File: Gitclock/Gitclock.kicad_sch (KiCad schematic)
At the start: 6 parts

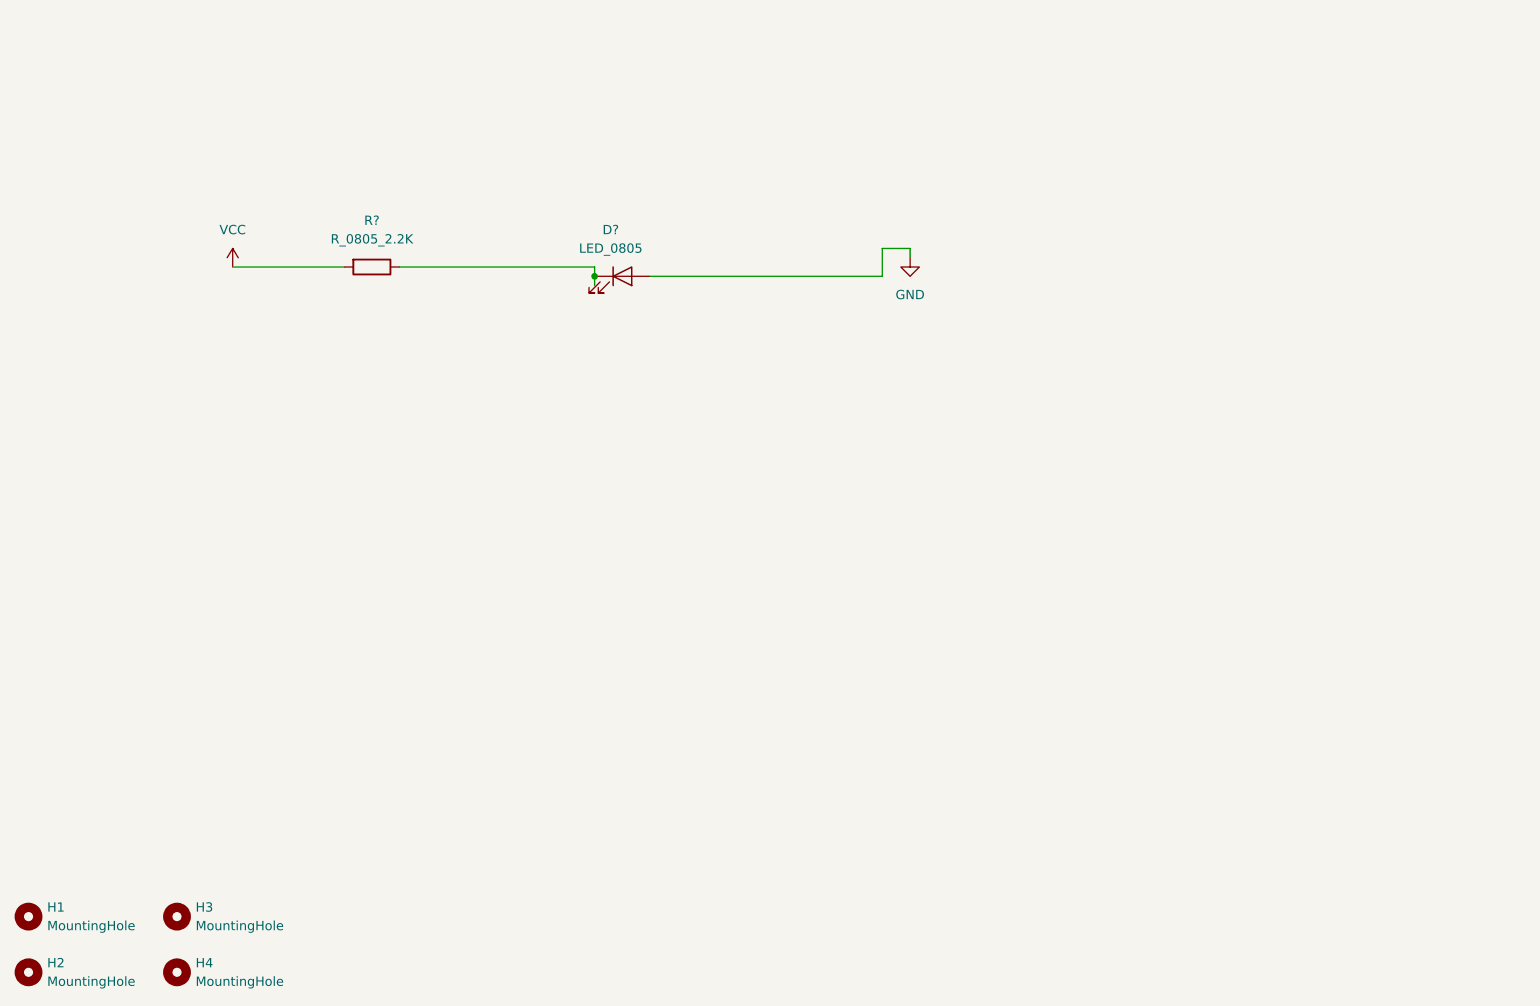
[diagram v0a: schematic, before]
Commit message: Week 2: Clock Schematic
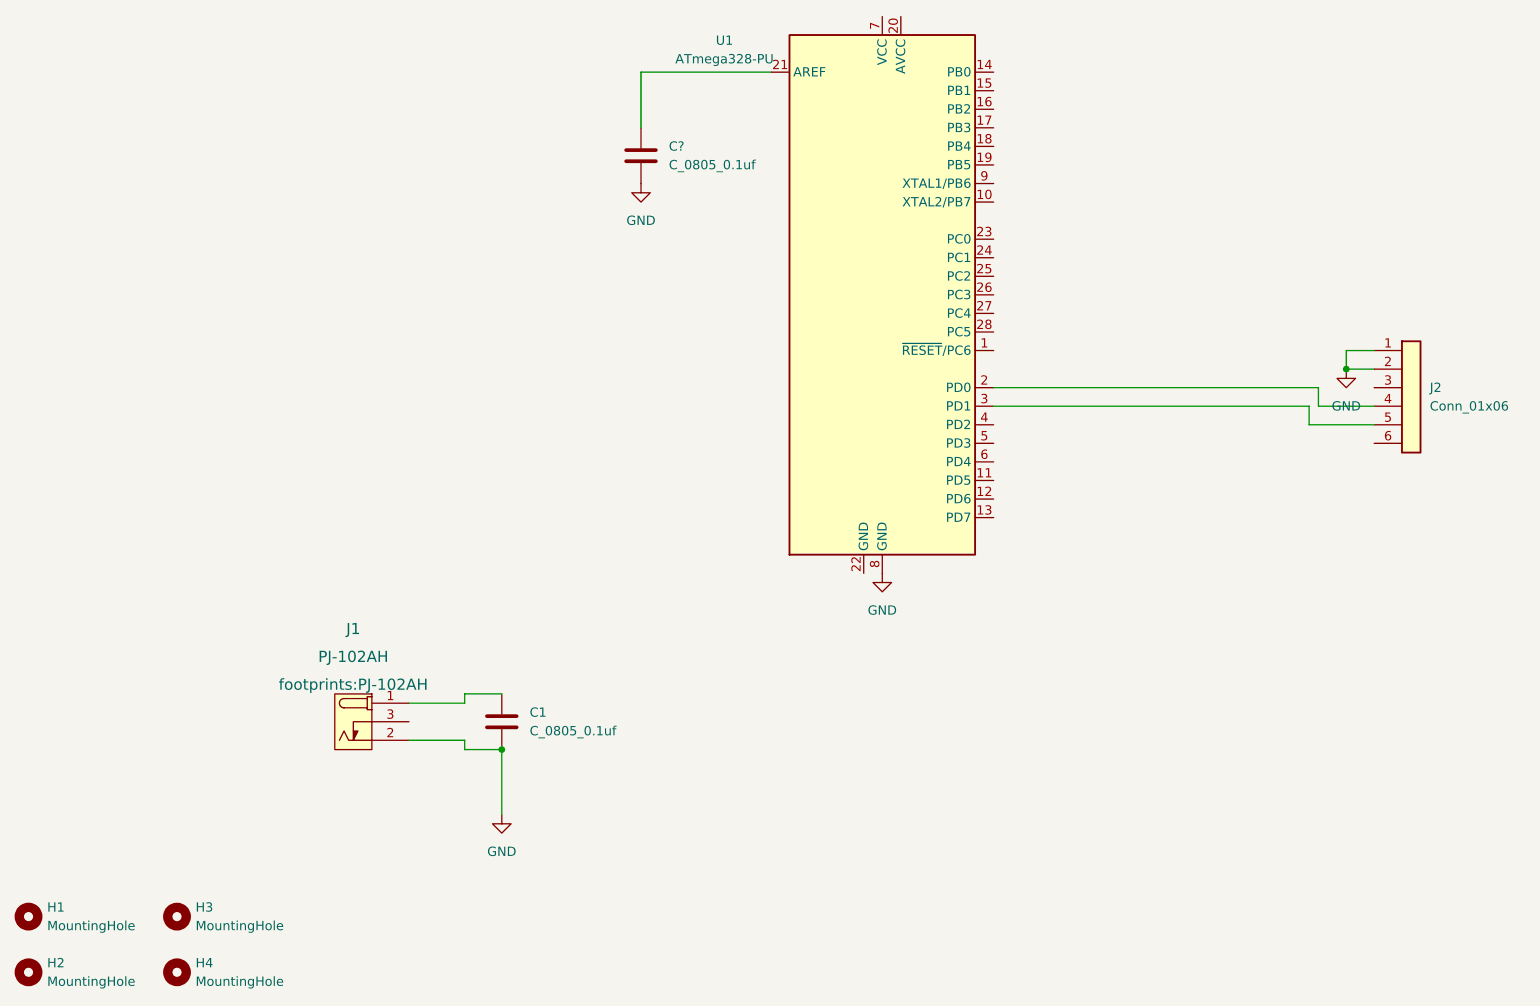
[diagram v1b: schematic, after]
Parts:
- removed D?: LED_0805, footprints:LED_0805_2012Metric, symbol HPS:LED_0805
- removed R?: R_0805_2.2K, footprints:R_0805_2012Metric, symbol HPS:R_0805_2.2K
- added C1, C?: C_0805_0.1uf, footprints:C_0805_2012Metric, symbol HPS:C_0805_0.1uf
- added J1: PJ-102AH, footprints:PJ-102AH, symbol HPS:PJ-102AH
- added J2: Conn_01x06, footprints:PinHeader_1x06_P2.54mm_Vertical, symbol HPS:Conn_01x06
- added U1: ATmega328-PU, footprints:DIP-28_W7.62mm, symbol HPS:ATmega328-PU
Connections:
- net GND: now also C1.2, C?.2, J1.2 (OUT), J2.1 (Pin_1), J2.2 (Pin_2), U1.8 (GND)
- new net: C1.1, J1.1 (POLE)
- new net: J2.4 (Pin_4), U1.2 (PD0)
- new net: J2.5 (Pin_5), U1.3 (PD1)
- new net: C?.1, U1.21 (AREF)
